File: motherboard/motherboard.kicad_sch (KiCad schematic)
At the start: 57 parts, among them U1 QT1481, U2 cap_touch, U3 cap_touch, k1 cap_touch, k10 cap_touch, k11 cap_touch, k12 cap_touch, k13 cap_touch, k14 cap_touch, k15 cap_touch, k2 cap_touch, k3 cap_touch, k4 cap_touch, k5 cap_touch, k6 cap_touch, k7 cap_touch, k8 cap_touch, k9 cap_touch

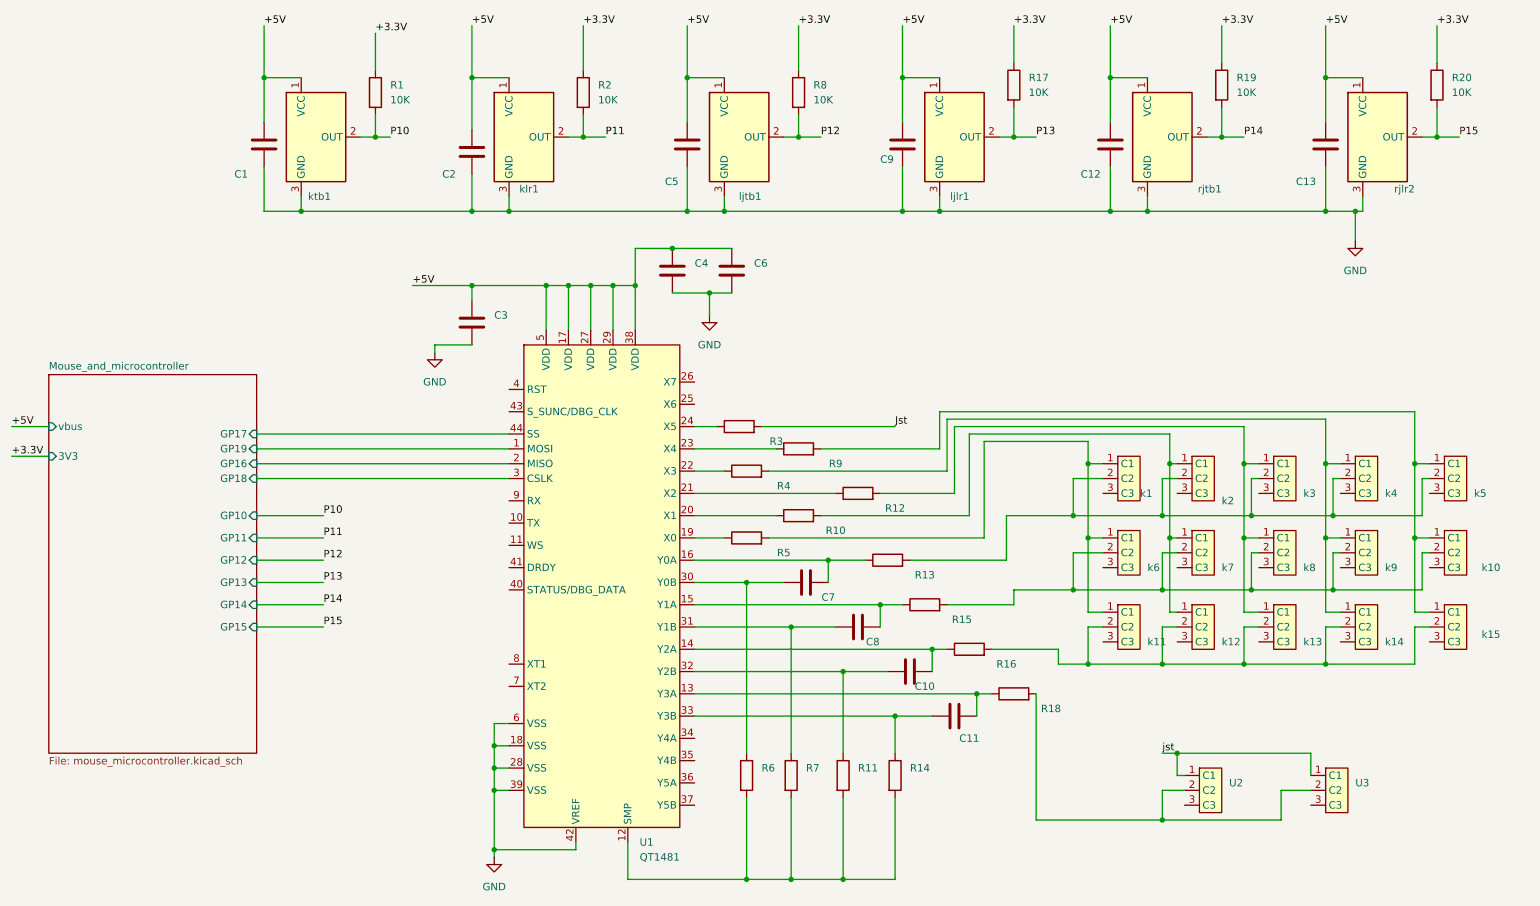
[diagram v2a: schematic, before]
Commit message: 3dmother
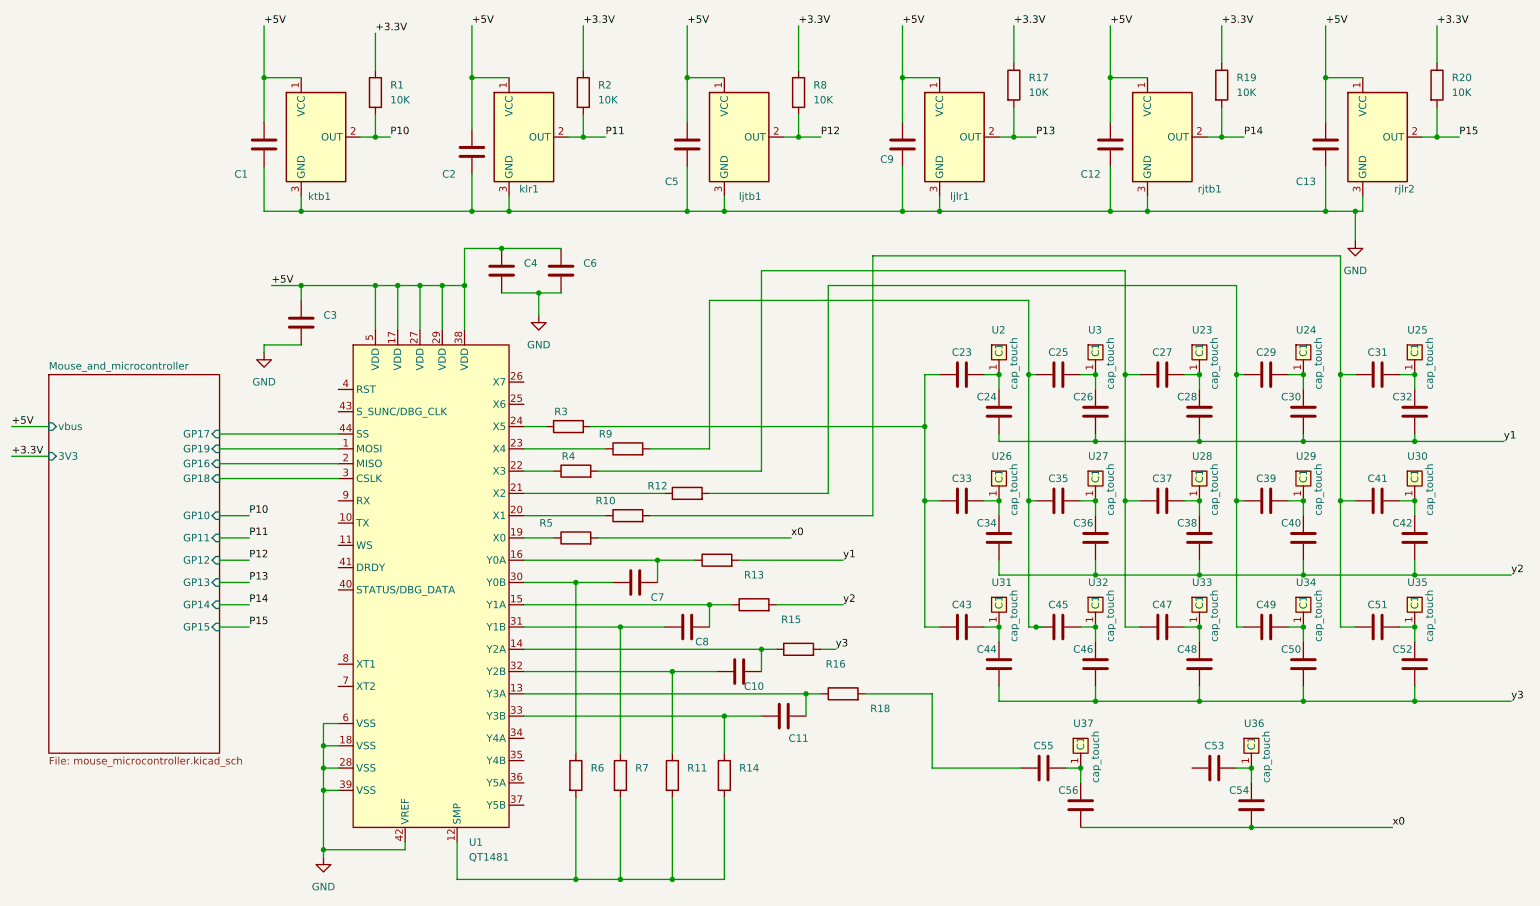
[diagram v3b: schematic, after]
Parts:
- removed k1, k10, k11, k12, k13, k14, k15, k2, k3, k4, k5, k6, k7, k8, k9: cap_touch, 42QT1481:cap_touch, symbol touch_keys:cap_touch
- added C23, C24, C25, C26, C27, C28, C29, C30, C31, C32, C33, C34, C35, C36, C37, C38, C39, C40, C41, C42, C43, C44, C45, C46, C47, C48, C49, C50, C51, C52, C53, C54, C55, C56: 50pF, Capacitor_Tantalum_SMD:CP_EIA-1608-10_AVX-L_Pad1.25x1.05mm_HandSolder, symbol Device:C
- added U23, U24, U25, U26, U27, U28, U29, U30, U31, U32, U33, U34, U35, U36, U37: cap_touch, 42QT1481:cap_touch, symbol touch_keys:cap_touch
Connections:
- net y3: now reaches R16.2
- net y3: now also C44.2, C46.2, C48.2, C50.2, C52.2
- net at R10.2: now also C31.1, C41.1, C51.1
- net y1: now reaches R13.2
- net y1: now also C24.2, C26.2, C28.2, C30.2, C32.2
- net at R12.2: now also C29.1, C39.1, C49.1
- net x0: now reaches R5.2
- net x0: now also C54.2, C56.2
- net at R4.2: now also C27.1, C37.1, C47.1
- net y2: now reaches R15.2
- net y2: now also C34.2, C36.2, C38.2, C40.2, C42.2
- net at R9.2: now also C25.1, C35.1, C45.1
- net Jst: no longer names the net of R3.2
- net Jst: now also C23.1, C33.1, C43.1
- net jst: no longer names the net of U2.1 (C1)
- net jst: now also C23.2, C24.1; no longer U3.1 (C1)
- new net: C47.2, C48.1, U33.1 (C1)
- new net: C39.2, C40.1, U29.1 (C1)
- new net: C31.2, C32.1, U25.1 (C1)
- new net: C33.2, C34.1, U26.1 (C1)
- new net: C37.2, C38.1, U28.1 (C1)
- new net: C35.2, C36.1, U27.1 (C1)
- new net: C53.2, C54.1, U36.1 (C1)
- new net: C43.2, C44.1, U31.1 (C1)
- new net: C27.2, C28.1, U23.1 (C1)
- new net: C55.1, R18.2
- new net: C55.2, C56.1, U37.1 (C1)
- new net: C41.2, C42.1, U30.1 (C1)
- new net: C45.2, C46.1, U32.1 (C1)
- new net: C51.2, C52.1, U35.1 (C1)
- new net: C29.2, C30.1, U24.1 (C1)
- new net: C49.2, C50.1, U34.1 (C1)
- new net: C25.2, C26.1, U3.1 (C1)
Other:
- moved on the sheet: C10, C11, C3, C4, C6, C7, C8, R10, R11, R12, R13, R14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
